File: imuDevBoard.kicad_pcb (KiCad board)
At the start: 2 copper layers, 33 x 26 mm, 39 parts, among them J1 USB_C_Receptacle_USB2.0_16P, SW1 SW_Push, SW2 SW_SPDT, U1 RP2350A, U2 W25Q128JVS, U3 TLV75533PDBV, U4 ICM-42688-P, Y1 Crystal_GND24, 12MHz

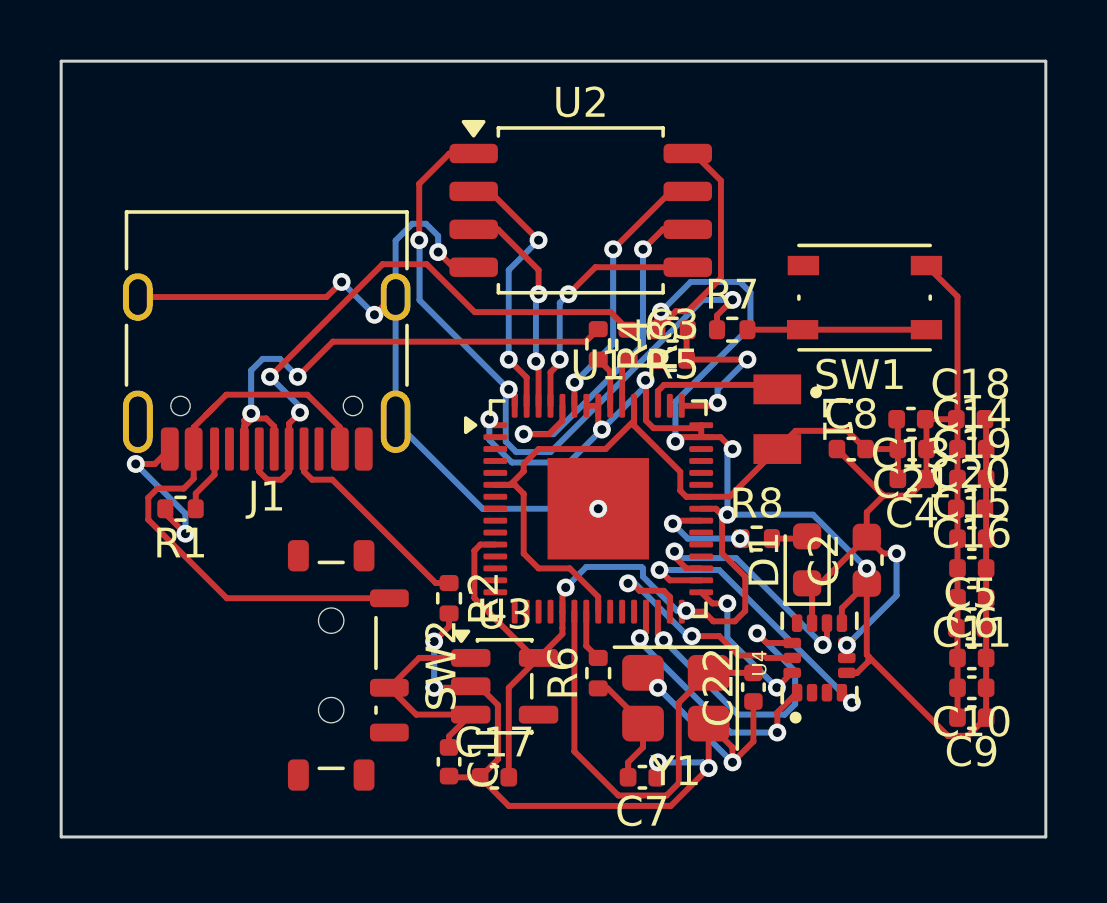
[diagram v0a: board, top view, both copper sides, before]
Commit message: fixed all errors on pcb
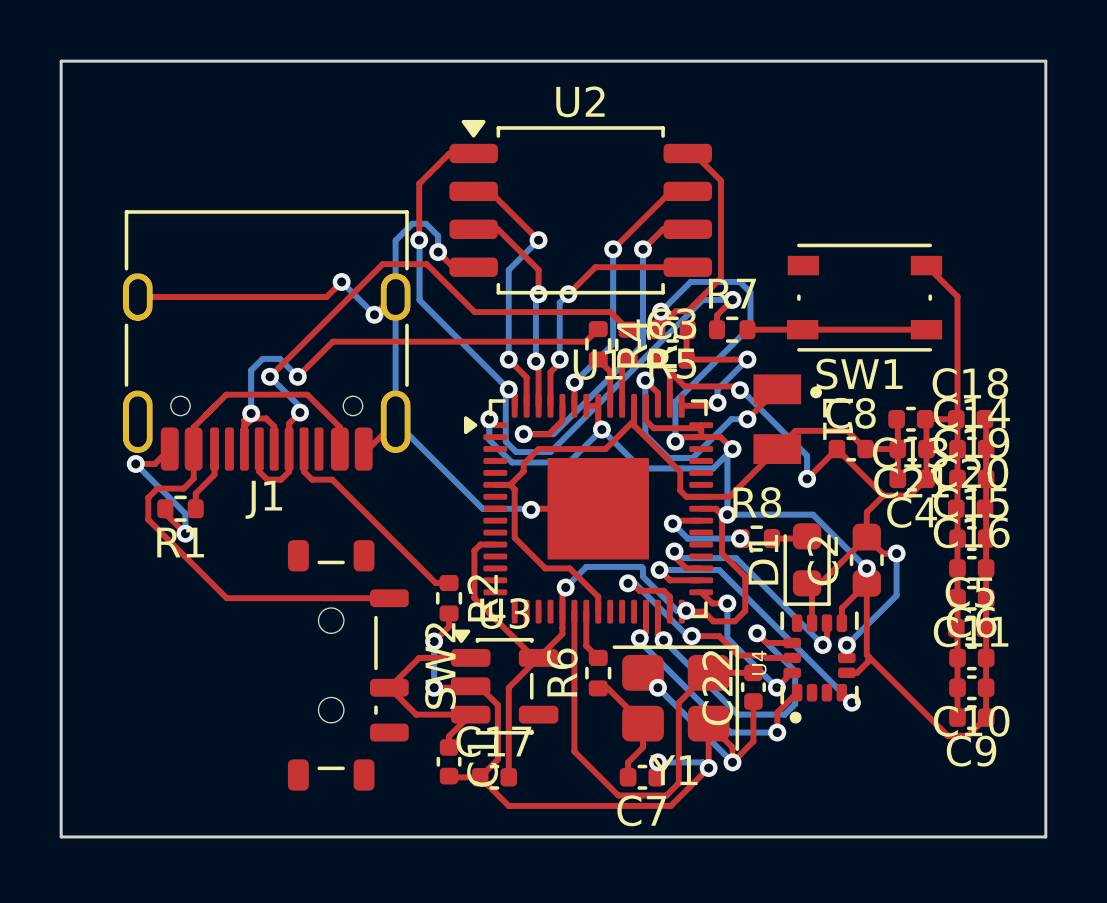
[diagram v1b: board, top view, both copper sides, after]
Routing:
- net GND: track 96.0 -> 107.8 mm, vias 14 -> 16
- net Net-(U1-VREG_LX): track 4.64 -> 8.75 mm, vias 0 -> 2
- net +3V3: track 86.4 -> 88.5 mm, vias 10 -> 9
- net Net-(U1-VREG_FB): track 26.9 -> 26.2 mm
